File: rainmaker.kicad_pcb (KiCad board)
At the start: 2 copper layers, 87.5 x 29.8 mm, 3 parts, among them J1 Micro_SD_Card, U1 C3 Pico

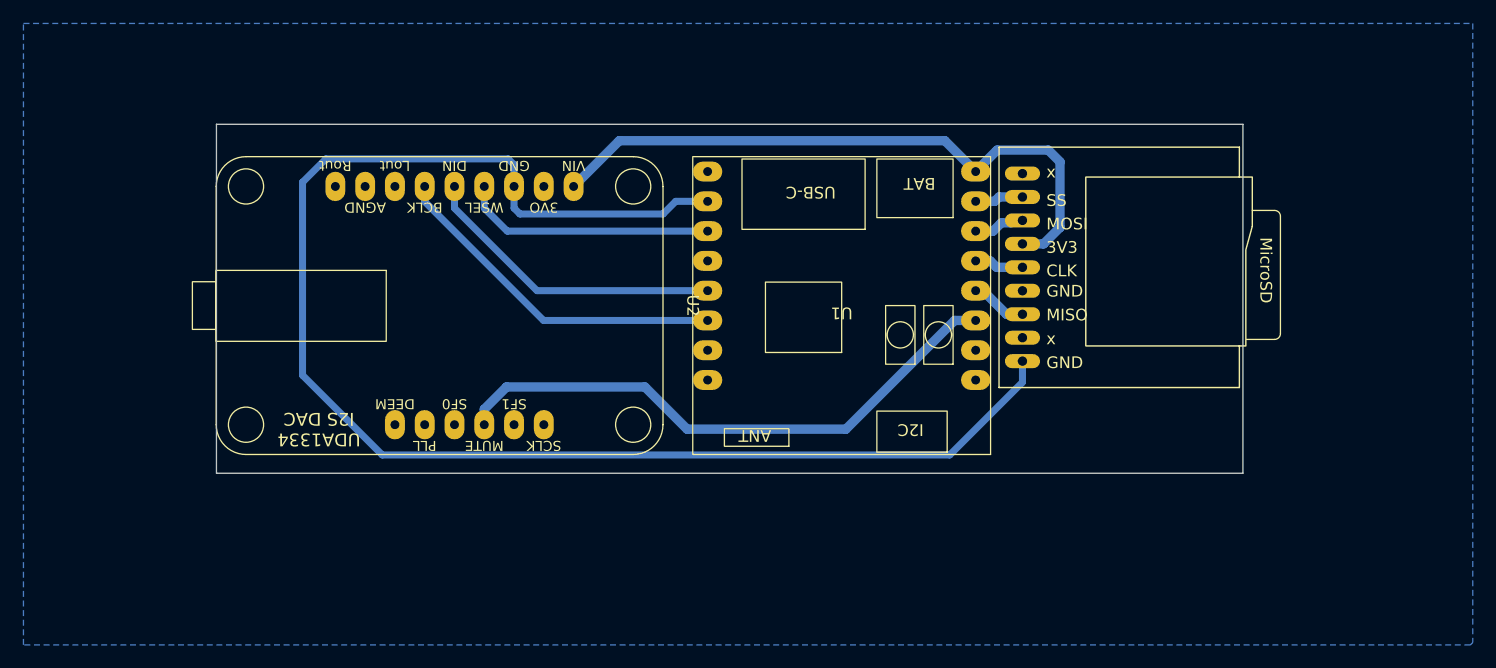
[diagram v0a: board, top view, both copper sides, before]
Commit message: Small pcb changes
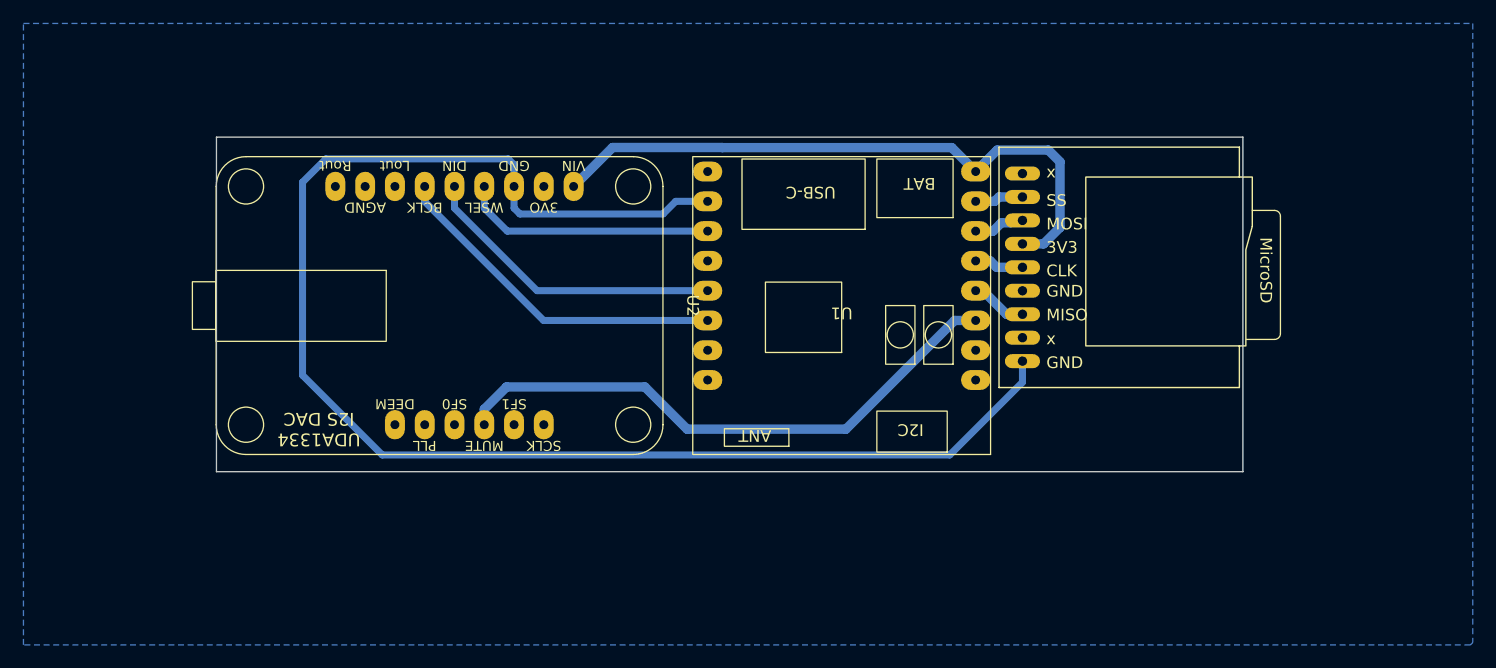
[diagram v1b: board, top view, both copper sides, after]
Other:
- board size 87.5 x 29.8 mm -> 87.5 x 28.5 mm
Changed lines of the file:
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@@
 	)
 	(gr_rect
-		(start 40.66 32.8)
-		(end 128.2 62.56)
+		(start 40.66 33.894482)
+		(end 128.2 62.427669)
 		(stroke
 			(width 0.05)
@@
 	)
 	(segment
+		(start 74.44 34.78)
+		(end 83.799138 34.78)
+		(width 0.8)
+		(layer "B.Cu")
+		(net 17)
+	)
+	(segment
 		(start 107.24 35)
 		(end 111.6 35)
@@
 	)
 	(segment
-		(start 75.02 34.2)
-		(end 102.78 34.2)
+		(start 71.12 38.1)
+		(end 74.44 34.78)
 		(width 0.8)
 		(layer "B.Cu")
@@
 	)
 	(segment
-		(start 102.78 34.2)
-		(end 105.41 36.83)
+		(start 83.80838 34.789242)
+		(end 103.369242 34.789242)
 		(width 0.8)
 		(layer "B.Cu")
@@
 	)
 	(segment
+		(start 83.799138 34.78)
+		(end 83.80838 34.789242)
+		(width 0.8)
+		(layer "B.Cu")
+		(net 17)
+	)
+	(segment
 		(start 111.2 43)
 		(end 109.4 43)
@@
 	)
 	(segment
-		(start 71.12 38.1)
-		(end 75.02 34.2)
+		(start 103.369242 34.789242)
+		(end 105.41 36.83)
 		(width 0.8)
 		(layer "B.Cu")
